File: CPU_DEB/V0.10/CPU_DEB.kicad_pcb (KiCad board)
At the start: 2 copper layers, 96.2 x 100.4 mm, 116 parts, among them J3 SIL1, J4 SIL1, J5 RJ12, J6 SIL1, J7 SIL1, K1 CONN_3, K2 CONN_3, K3 CONN_3, K4 CONN_3, K5 CONN_3, K6 CONN_3, K7 CONN_3, K8 CONN_2, P1 HE10-16, P10 CONN_2, P11 CONN_2, P2 CONN_4, P3 CONN_4, P4 CONN_4, P5 CONN_4, P6 CONN_4, P7 CONN_4, P8 CONN_2, P9 CONN_5, Q1 BSS123, Q2 BSS123, Q3 BSS123, Q4 BSS123, Q5 IRFL9014TRPBF, Q6 2N7002, SW2 SW_PUSH_SMALL, U1 PIC32MX795F512H, U2 74LVCC3245, U3 74LVCC3245, U4 PCA9306, U5 PCA9306, U6 74LVCC3245, U7 24C512, U8 LM75A, U9 PCF8563, X1 CRYSTAL1

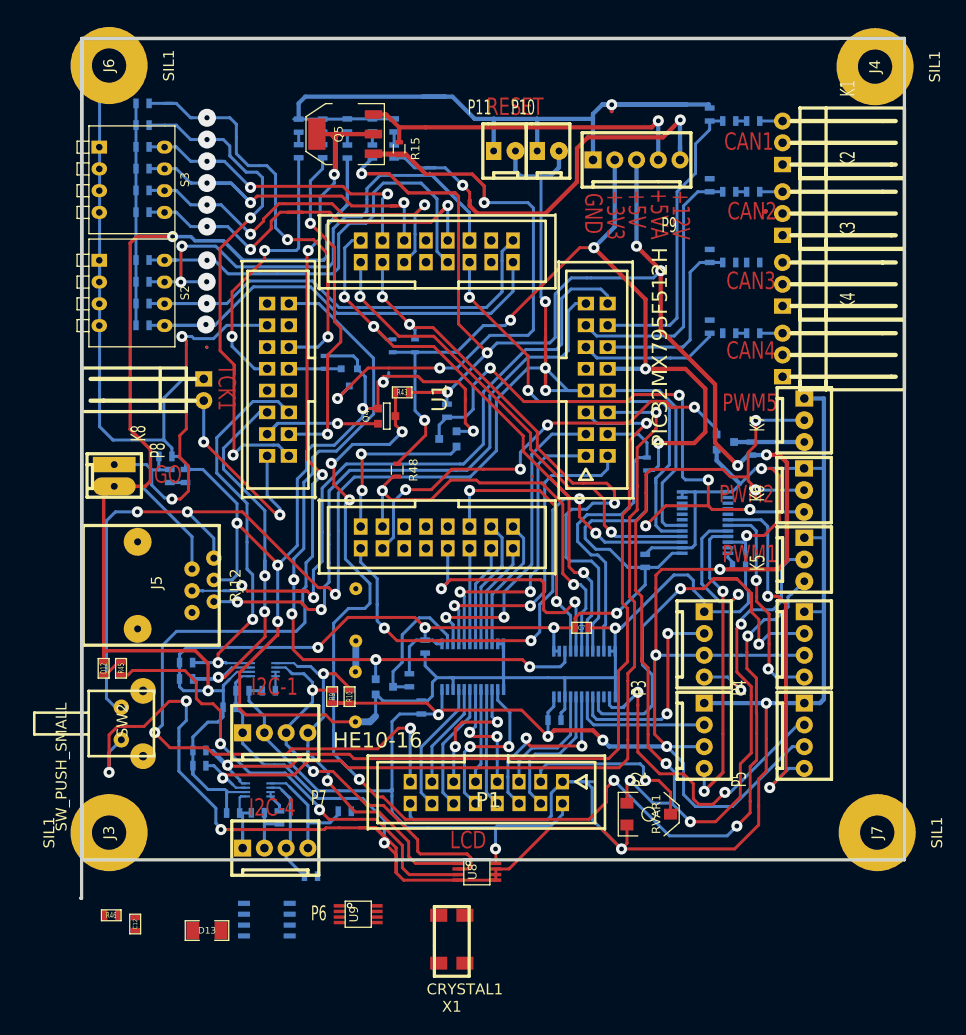
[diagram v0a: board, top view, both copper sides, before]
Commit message: INIT
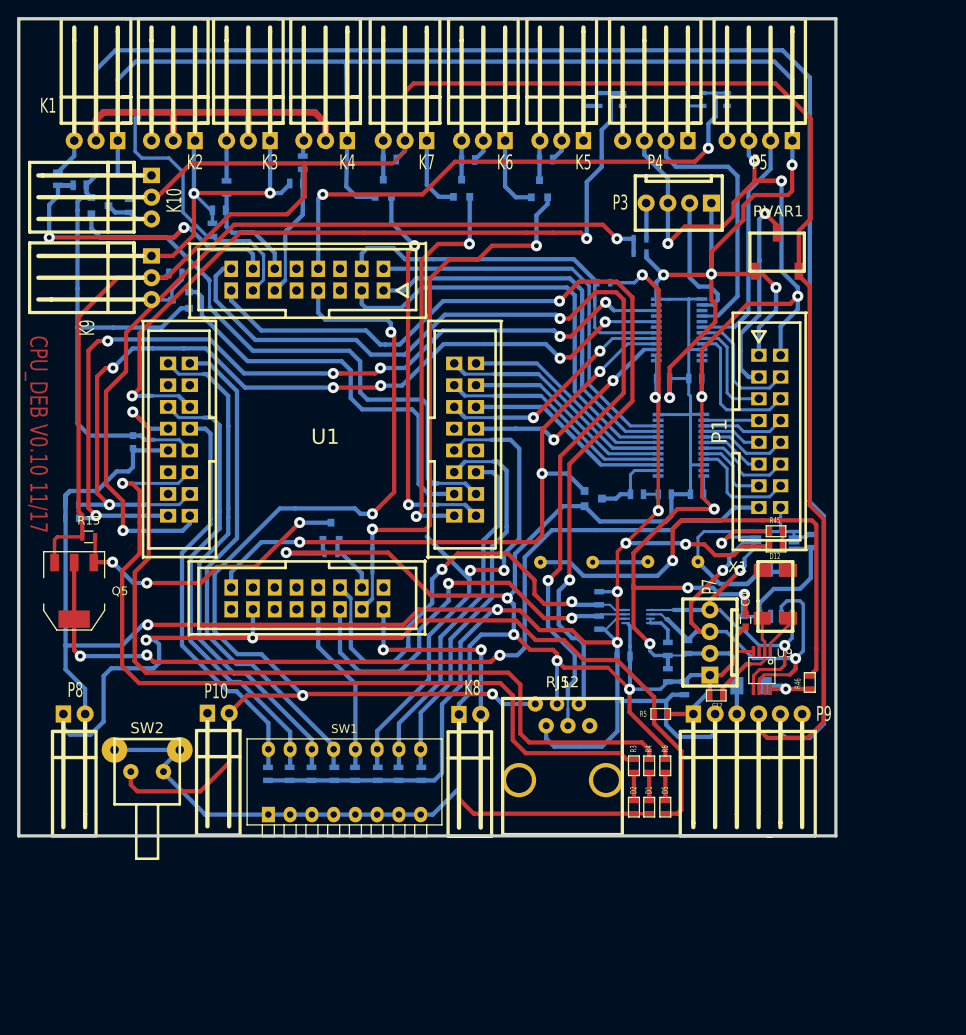
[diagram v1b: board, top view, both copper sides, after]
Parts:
- removed D10, D11, D3, D4, D7, D8, D9: LED, SM0603
- removed J3, J4, J6, J7: SIL1, COLONETTE
- removed P11: CONN_2, KK-2
- removed P2, P6: CONN_4, KK-4
- removed R39: 220k, SM0603_Resistor
- removed R44: 3..3k, SM0603_Resistor
- removed R49: 10k, Resistors_SMD:R_0603
- removed S2, S3: SW_DIP_x4, Buttons_Switches_ThroughHole:SW_DIP_x4_Piano
- removed U3: 74LVCC3245, SSOP24
- removed U5: PCA9306, VSSOP-8
- added K10: CONN_3, f4deb-mod-library:KK-3-H, F.Cu at (43.8, 77.7)
- added K9: CONN_3, f4deb-mod-library:KK-3-H, F.Cu at (43.8, 87.1)
- added Q7: BSS123, TO_SOT_Packages_SMD:SOT-23, B.Cu at (70.9, 71.6)
- added Q8: BSS123, TO_SOT_Packages_SMD:SOT-23, B.Cu at (47.2, 84.7)
- added SW1: SW_DIP_x08, Buttons_Switches_ThroughHole:SW_DIP_x8_Piano, F.Cu at (57.5, 144.7)
- C1: footprint SM0603_Capa -> Capacitors_SMD:C_0603
- C4: footprint SM0603_Capa -> Capacitors_SMD:C_0603; moved to F.Cu
- C7, D13, R10, R43, R48, R9, U8: moved to B.Cu
- D1, D2, D5, R3, R4, R5, R6: moved to F.Cu
- K5, K6, K7: footprint KK-3 -> f4deb-mod-library:KK-3-H
- P10, P8: footprint KK-2 -> f4deb-mod-library:KK-2-H
- P4, P5: footprint KK-4 -> f4deb-mod-library:KK-4-H
- P9: value CONN_5 -> CONN_6; footprint KK-5 -> f4deb-mod-library:KK-6-H
- Q1, Q2: footprint SOT23EBC -> TO_SOT_Packages_SMD:SOT-23
- Q4: footprint SOT23EBC -> TO_SOT_Packages_SMD:SOT-23; moved to B.Cu
- Q6: footprint SOT-23 -> TO_SOT_Packages_SMD:SOT-23
- R1: value 1k -> 4.7k
- R11, R12: value 2.1k -> 47k; footprint SM0603_Resistor -> CEN-PCB:SM0603_Resistor
- R13: value 1k -> 12k; footprint SM0603_Resistor -> Resistors_SMD:R_0603
- R14: value 1k -> 22k; footprint SM0603_Resistor -> Resistors_SMD:R_0603
- R16, R18: value 10K -> 12k; footprint SM0603_Resistor -> Resistors_SMD:R_0603
- R17, R19: value 10K -> 22k; footprint SM0603_Resistor -> Resistors_SMD:R_0603
- R2: value 330 -> 4.7k
- R20, R21, R22, R23, R24, R25: value 10K -> 47k; footprint SM0603_Resistor -> CEN-PCB:SM0603_Resistor
- RVAR1: footprint SMD_Packages:POT_SMD -> f4deb-mod-library:R-AJ-CMS
- U7: footprint SO8E -> Housings_SOIC:SOIC-8_3.9x4.9mm_Pitch1.27mm
- moved D2 88.7 mm to (100.1, 143.8), turned to 270 degrees
- moved D1 88.2 mm to (101.9, 143.8), turned to 270 degrees
- moved R46 85.9 mm to (120.7, 129.3), turned to 270 degrees
- moved K1 85.4 mm to (32.3, 66.0), turned to 0 degrees
- moved R13 83.7 mm to (100.8, 77.5)
- moved R25 82.1 mm to (67.6, 140.0), turned to 90 degrees
- moved R3 81.7 mm to (100.1, 139.0), turned to 270 degrees
- moved R4 81.2 mm to (101.9, 139.0), turned to 270 degrees
- moved D12 79.8 mm to (116.7, 113.4), turned to 0 degrees
- moved R30 78.6 mm to (32.9, 70.5), turned to 270 degrees
- moved R23 78.2 mm to (70.2, 140.0), turned to 90 degrees
- moved R45 78.1 mm to (116.7, 111.6), turned to 180 degrees
- moved Q2 78.0 mm to (37.8, 73.6), turned to 0 degrees
- moved R41 77.9 mm to (41.3, 73.7), turned to 270 degrees
- moved R24 77.1 mm to (57.4, 140.0), turned to 90 degrees
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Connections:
- net /5vto3v3/CONTRASTE renamed /CONT
- net /5vto3v3/SCL1-5V renamed /SCL1-5V
- net /5vto3v3/SDA1-5V renamed /SDA1-5V
- net /PIC32/RETROLCD renamed /RETRO
- J5 pad 7: Net-(J5-Pad7) -> GND
- J5 pad 8: Net-(J5-Pad8) -> GND
- K7 pad 3: /5vto3v3/OC5-5V -> /5vto3v3/OC3-5V
- P1 pad 4: /5vto3v3/BRS -> /BRS
- P1 pad 5: /5vto3v3/BRW -> /BRW
- P1 pad 6: /5vto3v3/BE -> /BE
- R1 pad 1: +5V -> +5VA
- R1 pad 2: Net-(D3-Pad1) -> /5vto3v3/OC3-5V
- R11 pad 2: /5vto3v3/SDA4 -> /PIC32/SW4
- R12 pad 2: /5vto3v3/SCL4 -> /PIC32/SW0
- R13 pad 1: Net-(P14-Pad1) -> /5vto3v3/U2RX-5V
- R13 pad 2: /5vto3v3/SCL4-5V -> /5vto3v3/U2RX
- R14 pad 1: Net-(P15-Pad1) -> /5vto3v3/U2RX
- R14 pad 2: /5vto3v3/SDA4-5V -> GND
- R16 pad 1: +3V3 -> /5vto3v3/U5RX-5V
- R16 pad 2: /PIC32/SW4 -> /5vto3v3/U5RX
- R17 pad 1: +3V3 -> /5vto3v3/U5RX
- R17 pad 2: /PIC32/SW5 -> GND
- R18 pad 1: +3V3 -> /5vto3v3/U6RX-5V
- R18 pad 2: /PIC32/SW6 -> /5vto3v3/U6RX
- R19 pad 1: +3V3 -> /5vto3v3/U6RX
- R19 pad 2: /PIC32/SW7 -> GND
- R2 pad 1: +3V3 -> +5VA
- R2 pad 2: Net-(D4-Pad1) -> /5vto3v3/OC4-5V
- R20 pad 2: /PIC32/SW8 -> /PIC32/SW5
- R21 pad 2: /PIC32/SW9 -> /PIC32/SW1
- R22 pad 2: /PIC32/SW10 -> /PIC32/SW6
- R23 pad 2: /PIC32/SW11 -> /PIC32/SW2
- R24 pad 2: /PIC32/SW12 -> /PIC32/SW7
- R25 pad 2: /PIC32/SW13 -> /PIC32/SW3
- R3 pad 1: /PIC32/PGED1 -> Net-(R3-Pad1)
- R30 pad 1: Net-(D7-Pad2) -> /PIC32/CAN1
- R31 pad 1: Net-(D8-Pad2) -> /PIC32/CAN2
- R32 pad 1: Net-(D9-Pad2) -> /PIC32/CAN3
- R33 pad 1: Net-(D10-Pad2) -> /PIC32/CAN4
- R4 pad 1: /PIC32/PGEC1 -> Net-(R4-Pad1)
- R40 pad 1: +5V -> +5VA
- R41 pad 1: +5V -> +5VA
- R43 pad 1: +5V -> +5VA
- R48 pad 2: /5vto3v3/U1TX -> /5vto3v3/U6TX
- R51 pad 2: /5vto3v3/U6TX -> /5vto3v3/U2TX
- RVAR1 pad 1: +5VA -> GND
- RVAR1 pad 3: GND -> +5VA
- U1 pad 1: /5vto3v3/D5 -> /5vto3v3/D1
- U1 pad 10: +3V3 -> Net-(U1-Pad10)
- U1 pad 2: /5vto3v3/D6 -> /5vto3v3/D0
- U1 pad 24: /PIC32/SW8 -> Net-(R4-Pad1)
- U1 pad 25: Net-(U1-Pad25) -> GND
- U1 pad 26: Net-(U1-Pad26) -> +3V3
- U1 pad 27: /PIC32/SW9 -> Net-(R3-Pad1)
- U1 pad 28: /PIC32/SW10 -> Net-(U1-Pad28)
- U1 pad 3: /5vto3v3/D7 -> /5vto3v3/D2
- U1 pad 30: /PIC32/SW11 -> Net-(U1-Pad30)
- U1 pad 37: /PIC32/SW13 -> Net-(U1-Pad37)
- U1 pad 47: /PIC32/SW12 -> Net-(U1-Pad47)
- U1 pad 5: /5vto3v3/SDA4 -> Net-(U1-Pad5)
- U1 pad 50: /5vto3v3/U1RX -> /5vto3v3/OC3
- U1 pad 51: /5vto3v3/U1TX -> /5vto3v3/OC4
- U1 pad 6: /5vto3v3/SCL4 -> Net-(U1-Pad6)
- U1 pad 60: /5vto3v3/D0 -> /5vto3v3/D7
- U1 pad 61: /5vto3v3/D1 -> /5vto3v3/D6
- U1 pad 62: /5vto3v3/D2 -> /5vto3v3/D5
- U1 pad 63: /5vto3v3/D3 -> /5vto3v3/D4
- U1 pad 64: /5vto3v3/D4 -> /5vto3v3/D3
- U1 pad 9: GND -> Net-(U1-Pad9)
- U2 pad 10: /5vto3v3/U6TX -> /5vto3v3/U2TX
- U2 pad 14: /5vto3v3/U6TX-5V -> /5vto3v3/U2TX-5V
- U2 pad 17: /5vto3v3/U2TX-5V -> Net-(U2-Pad17)
- U2 pad 18: /5vto3v3/U1TX-5V -> /5vto3v3/U6TX-5V
- U2 pad 19: /5vto3v3/BE -> /BRS
- U2 pad 20: /5vto3v3/BRS -> /BRW
- U2 pad 21: /5vto3v3/BRW -> /BE
- U2 pad 3: /5vto3v3/RW -> /5vto3v3/E
- U2 pad 4: /5vto3v3/RS -> /5vto3v3/RW
- U2 pad 5: /5vto3v3/E -> /5vto3v3/RS
- U2 pad 6: /5vto3v3/U1TX -> /5vto3v3/U6TX
- U2 pad 7: /5vto3v3/U2TX -> Net-(U2-Pad7)
- U6 pad 10: /5vto3v3/D3 -> /5vto3v3/D0
- U6 pad 14: /BD3 -> /BD0
- U6 pad 15: /BD4 -> /BD1
- U6 pad 16: /BD1 -> /BD2
- U6 pad 17: /BD2 -> /BD3
- U6 pad 18: /BD0 -> /BD4
- U6 pad 6: /5vto3v3/D0 -> /5vto3v3/D4
- U6 pad 7: /5vto3v3/D2 -> /5vto3v3/D3
- U6 pad 8: /5vto3v3/D1 -> /5vto3v3/D2
- U6 pad 9: /5vto3v3/D4 -> /5vto3v3/D1
- X1 pad 1: Net-(C12-Pad1) -> Net-(U9-Pad1)
- X1 pad 2: Net-(U9-Pad1) -> Net-(C12-Pad1)
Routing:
- net +12V: track 51.3 -> 217.0 mm, vias 2 -> 0
- net +3V3: track 453.6 -> 289.0 mm, vias 11 -> 9
- net +5V: track 348.5 -> 185.2 mm, vias 14 -> 9
- net /5vto3v3/OC1-5V: track 143.8 -> 4.63 mm, vias 7 -> 0
- net Net-(R4-Pad1): track 0.00 -> 105.4 mm, vias 0 -> 1
- net /5vto3v3/SDA4: track 104.0 -> 0.00 mm, vias 2 -> 0
- net /5vto3v3/SCL4: track 102.9 -> 0.00 mm, vias 2 -> 0
- net +5VA: track 168.0 -> 270.4 mm, vias 7 -> 0
- net Net-(R3-Pad1): track 0.00 -> 99.3 mm, vias 0 -> 1
- net /5vto3v3/U2RX: track 56.2 -> 142.7 mm
- net /5vto3v3/OC2-5V: track 75.2 -> 4.56 mm, vias 5 -> 0
- net /5vto3v3/U1RX: track 63.6 -> 0.00 mm, vias 4 -> 0
- net /PIC32/GO: track 45.1 -> 107.9 mm
- net /PIC32/SW2: track 0.00 -> 62.6 mm, vias 0 -> 2
- net /PIC32/SW12: track 59.1 -> 0.00 mm, vias 3 -> 0
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- added copper zone on B.Cu, net GND
- added copper zone on F.Cu, net GND
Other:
- board size 96.2 x 100.4 mm -> 95.4 x 95.4 mm
- board text added: "CPU_DEB V0.10 11/17"
- board text removed: "+12V"
- board text removed: "+3V3"
- board text removed: "+5V"
- board text removed: "+5VA"
- board text removed: "CAN1"
- board text removed: "CAN2"
- board text removed: "CAN3"
- board text removed: "CAN4"
- board text removed: "GND"
- board text removed: "GO"
- board text removed: "I2C-1"
- board text removed: "I2C-4"
- board text removed: "LCD"
- board text removed: "PWM1"
- board text removed: "PWM2"
- board text removed: "PWM5"
- board text removed: "RESET"
- board text removed: "TCK1"
